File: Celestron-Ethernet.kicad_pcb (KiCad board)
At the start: 4 copper layers, 90.4 x 33.3 mm, 59 parts, among them J2 6P6C, J3 RJ45_Abracon_ARJP11A-MASA-B-A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, U2 LP2985-5.0, U3 LP2985-3.3

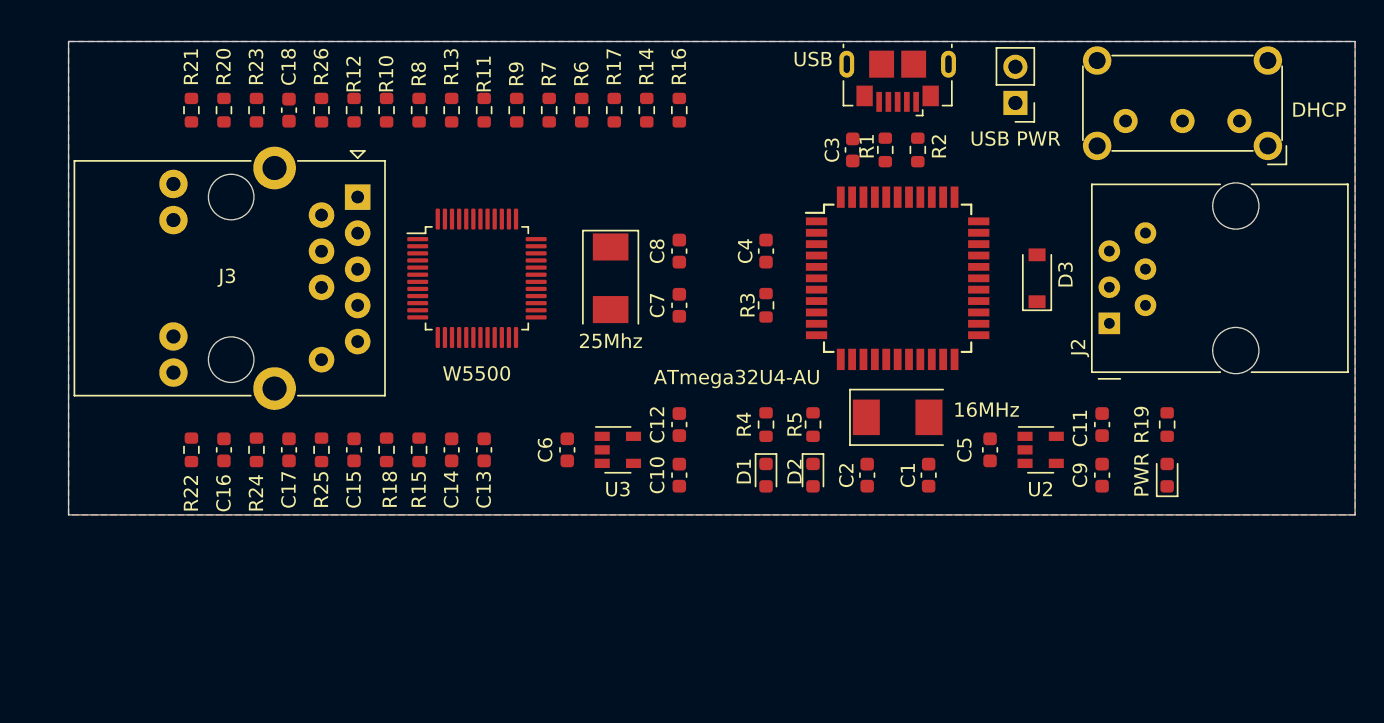
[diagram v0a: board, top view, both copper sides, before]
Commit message: Initial routing
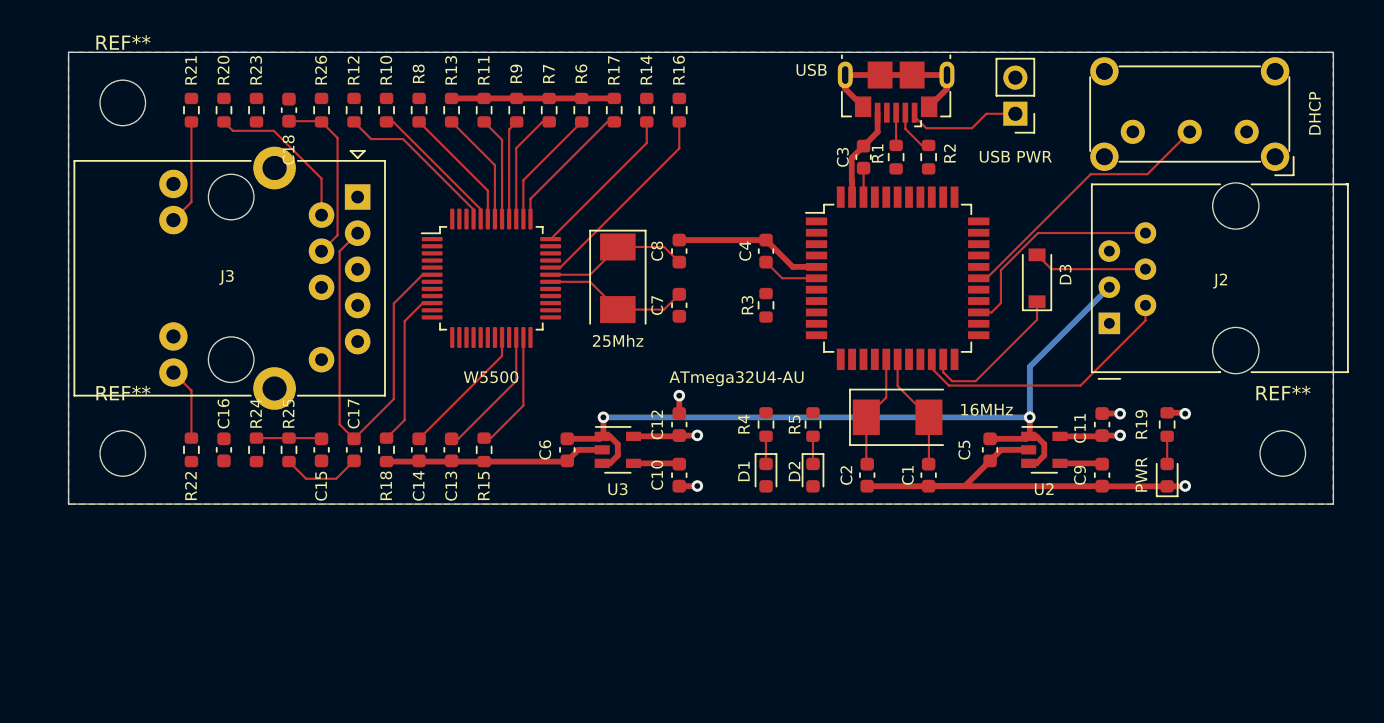
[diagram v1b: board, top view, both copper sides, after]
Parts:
- added REF**: MountingHole_3.2mm_M3, MountingHole:MountingHole_3.2mm_M3, F.Cu at (189.7, 97.5)
- added REF**: MountingHole_3.2mm_M3, MountingHole:MountingHole_3.2mm_M3, F.Cu at (108.2, 97.5)
- added REF**: MountingHole_3.2mm_M3, MountingHole:MountingHole_3.2mm_M3, F.Cu at (108.2, 72.9)
- moved R15 4.57 mm to (133.6, 97.3)
- moved C17 4.57 mm to (124.5, 97.3), turned to 270 degrees
- moved C13 2.29 mm to (131.3, 97.3)
- moved C14 2.29 mm to (129.0, 97.3)
- moved R25 2.29 mm to (119.9, 97.3), turned to 270 degrees
- moved C15 2.29 mm to (122.2, 97.3)
- moved W5500 1.02 mm to (134.1, 85.2)
- moved DHCP 0.92 mm to (187.2, 74.9)
- moved C3 0.92 mm to (160.3, 76.7)
- moved R1 0.92 mm to (162.6, 76.7)
- moved R2 0.92 mm to (164.8, 76.7)
- moved USB 0.77 mm to (162.6, 72.1)
- moved USB PWR 0.76 mm to (170.9, 73.7)
- moved 25Mhz 0.51 mm to (143.0, 85.2)
- moved U2 0.25 mm to (173.0, 97.3)
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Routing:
- net GND: track 0.00 -> 78.3 mm, vias 0 -> 4
- net Net-(C5-Pad1): track 0.00 -> 56.4 mm, vias 0 -> 2
- net Net-(C17-Pad1): track 0.00 -> 29.6 mm
- net Net-(SW1-Pad2): track 0.00 -> 19.8 mm
- net Net-(J2-Pad2): track 0.00 -> 19.1 mm
- net Net-(J2-Pad6): track 0.00 -> 15.4 mm
- net Net-(R16-Pad2): track 0.00 -> 14.4 mm
- net Net-(J1-Pad6): track 0.00 -> 12.6 mm
- net Net-(C18-Pad2): track 0.00 -> 12.3 mm
- net Net-(R12-Pad2): track 0.00 -> 11.6 mm
- net Net-(R18-Pad2): track 0.00 -> 11.2 mm
- net Net-(J3-Pad2): track 0.00 -> 11.1 mm
- net Net-(R14-Pad2): track 0.00 -> 11.0 mm
- net Net-(D3-Pad1): track 0.00 -> 10.8 mm
- net Net-(C7-Pad2): track 0.00 -> 10.3 mm
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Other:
- board size 90.4 x 33.3 mm -> 88.9 x 31.8 mm
- net class Default: clearance 0.2 -> 0.1524; trace_width 0.25 -> 0.1524; via_dia 0.8 -> 0.4572; via_drill 0.4 -> 0.2286
- net class Power added: clearance 0.1524, trace_width 0.4064, via_dia 0.8128, via_drill 0.4064
- rule pad_to_mask_clearance: 0 -> 0.0508
- rule trace_clearance: 0.2 -> 0.1524
- rule trace_min: 0.2 -> 0.1524
- rule via_min_drill: 0.3 -> 0.2286
- rule via_min_size: 0.4 -> 0.4572

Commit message: bypass caps
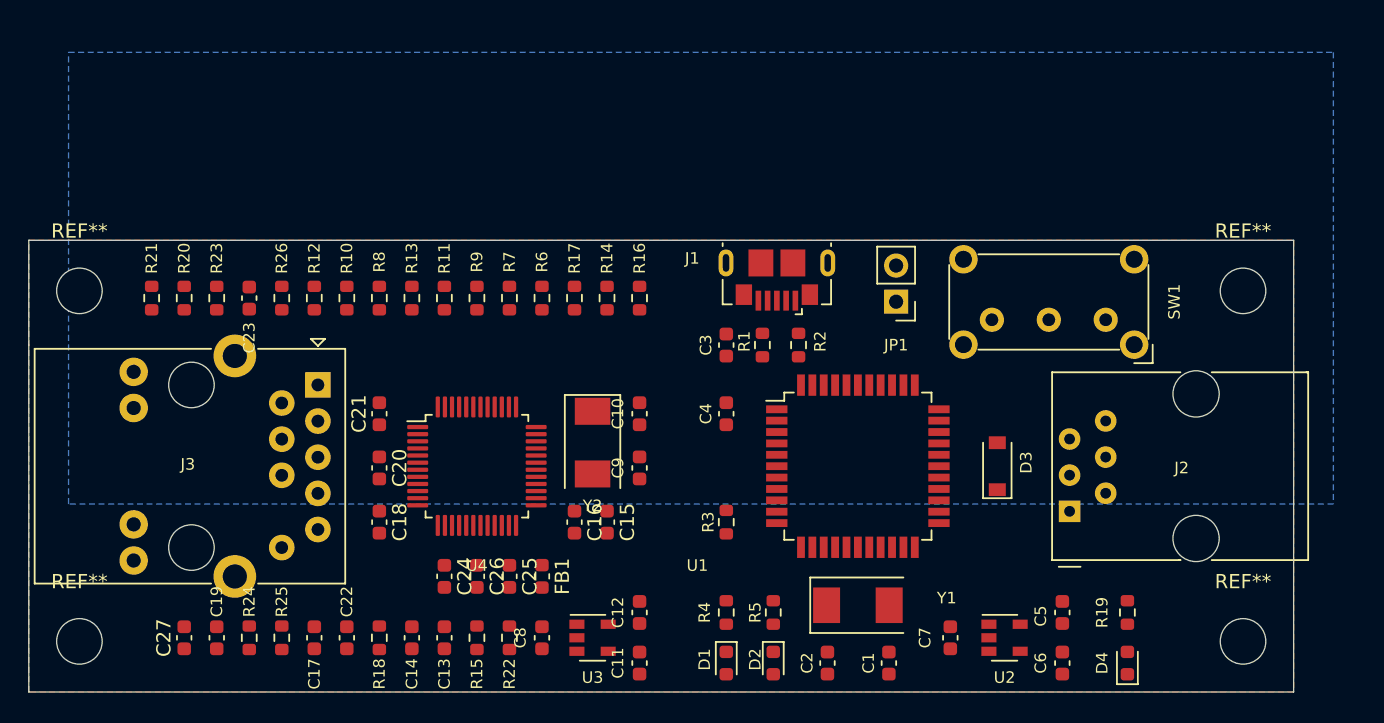
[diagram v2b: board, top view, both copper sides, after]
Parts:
- removed the REF** at (108.2, 72.9)
- added C19: 6.8nF, Capacitor_SMD:C_0603_1608Metric, F.Cu at (114.8, 110.5)
- added C20: 100nF, Capacitor_SMD:C_0603_1608Metric, F.Cu at (126.2, 98.6)
- added C21: 100nF, Capacitor_SMD:C_0603_1608Metric, F.Cu at (126.2, 94.7)
- added C22: 6.8nF, Capacitor_SMD:C_0603_1608Metric, F.Cu at (124.0, 110.5)
- added C23: 22nF, Capacitor_SMD:C_0603_1608Metric, F.Cu at (117.1, 86.6)
- added C24: 100nF, Capacitor_SMD:C_0603_1608Metric, F.Cu at (130.8, 106.2)
- added C25: 100nF, Capacitor_SMD:C_0603_1608Metric, F.Cu at (135.4, 106.2)
- added C26: 100nF, Capacitor_SMD:C_0603_1608Metric, F.Cu at (133.1, 106.2)
- added C27: 1nF/2KV, Capacitor_SMD:C_0603_1608Metric, F.Cu at (112.5, 110.5)
- added FB1: HH-1M1608-121JT, Inductor_SMD:L_0603_1608Metric, F.Cu at (137.7, 106.2)
- added REF**: MountingHole_3.2mm_M3, MountingHole:MountingHole_3.2mm_M3, F.Cu at (186.9, 86.1)
- added REF**: MountingHole_3.2mm_M3, MountingHole:MountingHole_3.2mm_M3, F.Cu at (105.2, 86.1)
- C15: value 10nF -> 10uF
- C16: value 6.8nF -> 100nF
- C17: value 6.8nF -> 10nF
- C18: value 22nF -> 100nF
- JP1: renamed from USB PWR
- R18: value 12K4 -> 12.4K
- moved C18 29.6 mm to (126.2, 102.4)
- moved R22 26.0 mm to (135.4, 110.5)
- moved C16 25.2 mm to (140.0, 102.4)
- moved C15 20.7 mm to (142.2, 102.4), turned to 270 degrees
- moved SW1 16.5 mm to (177.3, 88.1)
- moved C3 16.4 mm to (150.6, 89.9)
- moved R1 16.2 mm to (153.2, 89.9)
- moved R2 16.1 mm to (155.7, 89.9)
- moved J1 15.6 mm to (154.2, 85.3)
- moved JP1 15.6 mm to (162.6, 86.9)
- moved R3 15.5 mm to (150.6, 102.4)
- moved REF** 13.6 mm to (105.2, 110.7)
- moved D3 13.5 mm to (169.7, 98.4)
- moved U1 13.5 mm to (159.9, 98.4)
- moved C1 13.5 mm to (162.1, 112.3)
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- renumbered C8 to C10, C10 to C11, C11 to C5, C9 to C6, C5 to C7, C6 to C8, C7 to C9, PWR to D4, USB to J1, DHCP to SW1, ATmega32U4-AU to U1, W5500 to U4, 16MHz to Y1, 25Mhz to Y2
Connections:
- net Net-(C5-Pad1) renamed /12V
- C15 pad 1: GND -> +3V3
- C15 pad 2: Net-(C15-Pad2) -> GND
- C16 pad 1: Net-(C16-Pad1) -> +3V3
- C16 pad 2: Net-(C16-Pad2) -> GND
- C17 pad 1: Net-(C17-Pad1) -> GND
- C18 pad 1: GND -> +3.3VA
- C18 pad 2: Net-(C18-Pad2) -> GND
- J3 pad 15: Net-(J3-Pad15) -> GNDPWR
- J3 pad 3: Net-(C17-Pad1) -> Net-(C22-Pad1)
- J3 pad 4: Net-(C18-Pad2) -> Net-(C23-Pad2)
- J3 pad 5: Net-(C15-Pad2) -> Net-(C17-Pad2)
- J3 pad 6: Net-(C16-Pad1) -> Net-(C19-Pad1)
- R24 pad 1: Net-(C15-Pad2) -> Net-(C17-Pad2)
- R24 pad 2: Net-(C16-Pad2) -> Net-(C19-Pad2)
- R25 pad 1: Net-(C15-Pad2) -> Net-(C17-Pad2)
- R25 pad 2: Net-(C17-Pad2) -> Net-(C22-Pad2)
- R26 pad 1: Net-(C18-Pad2) -> Net-(C23-Pad2)
- U4 pad 11: +3V3 -> +3.3VA
- U4 pad 15: +3V3 -> +3.3VA
- U4 pad 17: +3V3 -> +3.3VA
- U4 pad 21: +3V3 -> +3.3VA
- U4 pad 4: +3V3 -> +3.3VA
- U4 pad 5: Net-(C16-Pad1) -> Net-(C19-Pad1)
- U4 pad 6: Net-(C17-Pad1) -> Net-(C22-Pad1)
- U4 pad 8: +3V3 -> +3.3VA
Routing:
- net GND: track 78.3 -> 0.00 mm, vias 4 -> 0
- net /12V: track 56.4 -> 0.00 mm, vias 2 -> 0
- net Net-(C17-Pad1): track 29.6 -> 0.00 mm
- net Net-(SW1-Pad2): track 19.8 -> 0.00 mm
- net Net-(J2-Pad2): track 19.1 -> 0.00 mm
- net Net-(J2-Pad6): track 15.4 -> 0.00 mm
- net Net-(R16-Pad2): track 14.4 -> 0.00 mm
- net Net-(J1-Pad6): track 12.6 -> 0.00 mm
- net Net-(C18-Pad2): track 12.3 -> 0.00 mm
- net Net-(R12-Pad2): track 11.6 -> 0.00 mm
- net Net-(R18-Pad2): track 11.2 -> 0.00 mm
- net Net-(J3-Pad2): track 11.1 -> 0.00 mm
- net Net-(R14-Pad2): track 11.0 -> 0.00 mm
- net Net-(D3-Pad1): track 10.8 -> 0.00 mm
- net Net-(C9-Pad2): track 10.3 -> 0.00 mm
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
